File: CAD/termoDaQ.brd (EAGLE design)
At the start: 99.1 x 72.4 mm, 72 parts, among them J1 TEST SUPPLY, J10 POTENTIOMETER, J11 SUPPLY, J12 SUPPLY, J13 V+, J14 B+, J15 VCC, J16 V-, J17 B-, J18 GND, J19 SUPPLY, J2 ADC, J20 VCC, J21 CONN_26X2, J22 CONN_26X2, J23 CONN_26X2, J24 CONN_20X2, J25 FEMALE 2x3, J3 GPS, J4 SERIAL, J5 GPS ON/OF, J6 INT, J7 MPX, J8 SD, J9 EN, T1 2N2222, U1 328P, U2 DS18B20, U3 TINY85-20-DIP, Y1 16MHz, Y2 16MHz

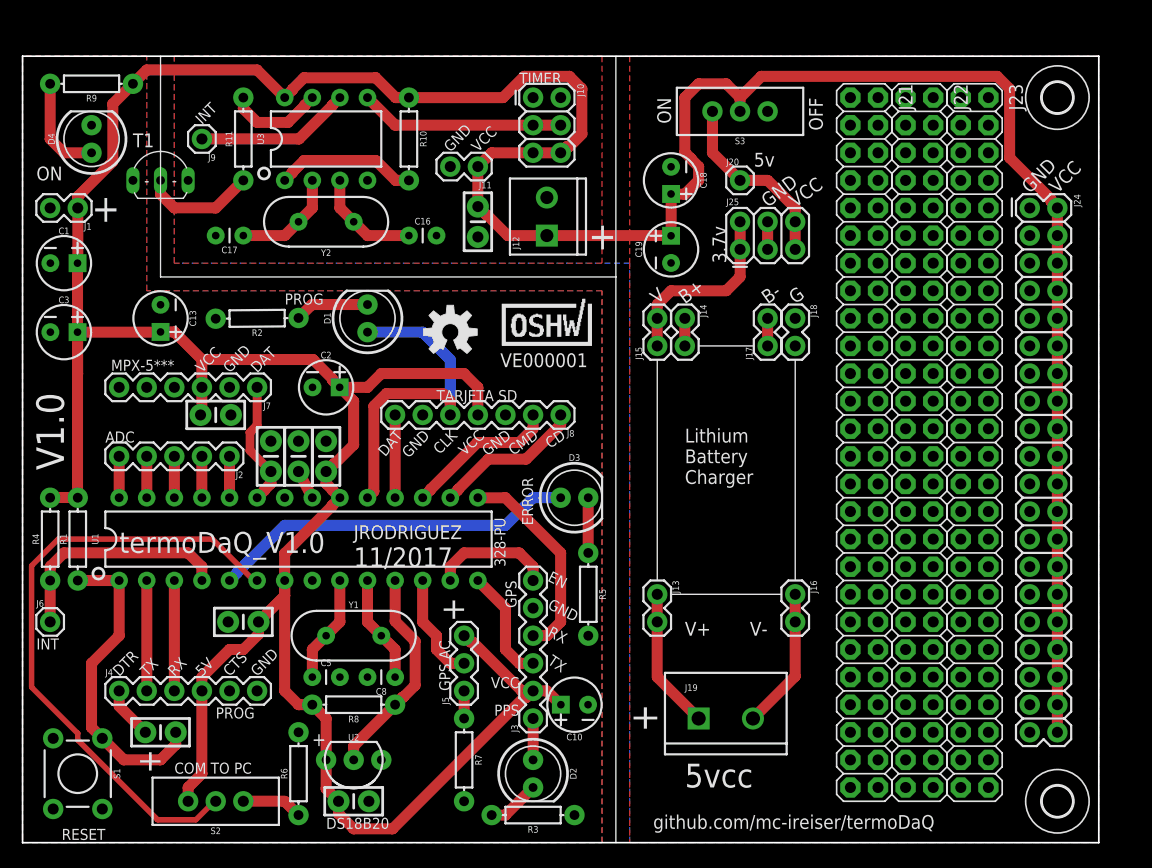
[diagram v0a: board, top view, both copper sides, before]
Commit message: Source files, Update
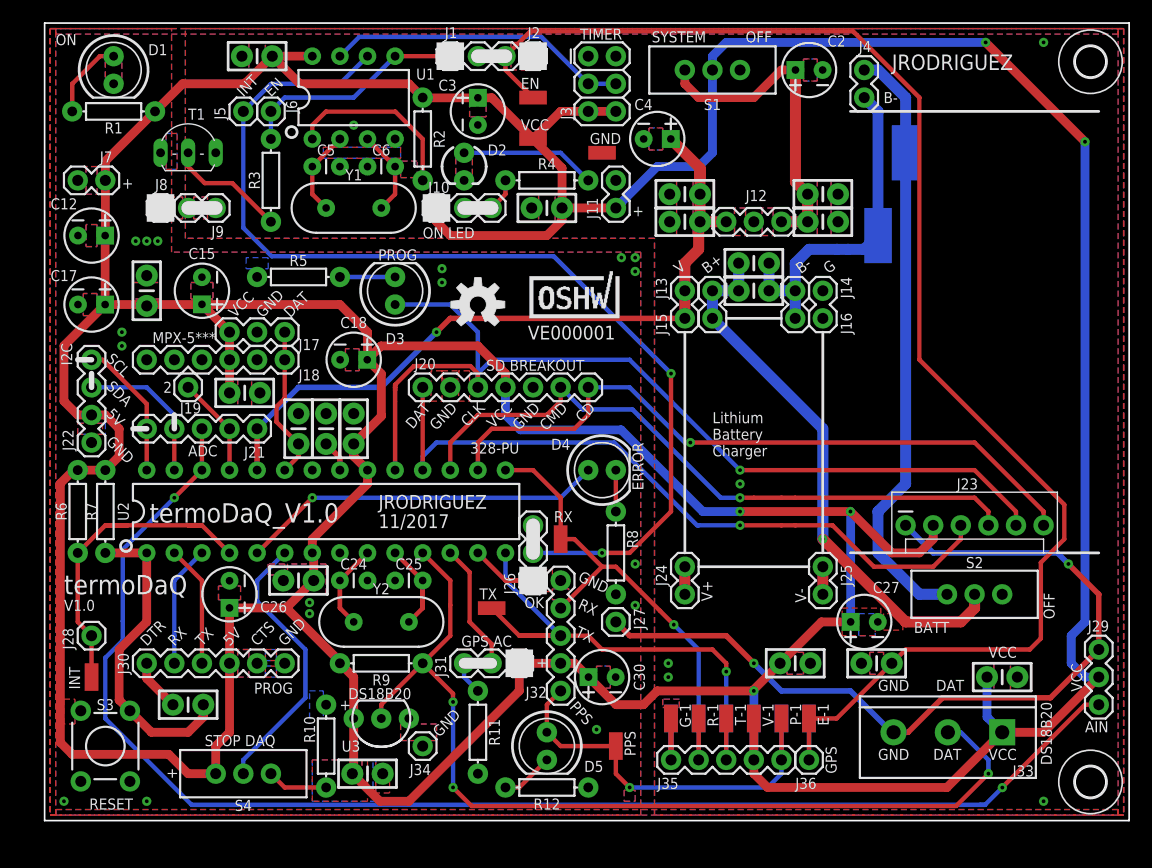
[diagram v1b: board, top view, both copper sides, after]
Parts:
- added B+: B+, wirepad:SMD2,54-5,08
- added B-: B-, wirepad:SMD2,54-5,08
- added C20, C21, C22, C23, C28, C29, C31, C32, C33: 0.1uF, SparkFun-Capacitors:CAP-PTH-SMALL-KIT
- added C24, C25: 22pF, SparkFun-Capacitors:CAP-PTH-2.54
- added C26, C27, C30: 10uF, SparkFun-Capacitors:CPOL-RADIAL-2.5MM-5MM
- added D5: PPS, SparkFun-LED:LED_5MM
- added E-1, E-2, EN: EN GPS, wirepad:SMD1,27-2,54
- added G-1, G-2: G, wirepad:SMD1,27-2,54
- added GND: GND, wirepad:SMD1,27-2,54
- added INT: INT1, wirepad:SMD1,27-2,54
- added J26: OK, SparkFun-Connectors:1X03
- added J27: GND2, SparkFun-Connectors:1X01
- added J28: INT1, SparkFun-Connectors:1X01
- added J29: AIN, SparkFun-Connectors:1X03
- added J30: SERIAL, SparkFun-Connectors:1X06
- added J31: GPS ON/OF, SparkFun-Connectors:1X03
- added J32, J35: GPS, SparkFun-Connectors:1X05
- added J33: TERMINAL SONDA, SparkFun-Connectors:SCREWTERMINAL-5MM-3
- added J34: GND, SparkFun-Connectors:1X01
- added J36: EN, SparkFun-Connectors:1X01
- added P-1, P-2: P, wirepad:SMD1,27-2,54
- added PPS: PPS, wirepad:SMD1,27-2,54
- added R-1, R-2: R, wirepad:SMD1,27-2,54
- added R12: 330, SparkFun-Resistors:AXIAL-0.3
- added RX: RX, wirepad:SMD1,27-2,54
- added S4: STREAM, SparkFun-Switches:SWITCH_SPDT_PTH_11.6X4.0MM
- added T-1, T-2: T, wirepad:SMD1,27-2,54
- added TX: TX, wirepad:SMD1,27-2,54
- added U$100: (no value), SparkFun-Aesthetics:OSHW-LOGO-M
- added U$101: (no value), OSHWA:CERT-SMALL-SILK
- added V-1, V-2: V, wirepad:SMD1,27-2,54
- added VCC: VCC, wirepad:SMD1,27-2,54
- C1, C10, C13, C19: value 22uF -> 0.1uF; device SparkFun-Capacitors:CPOL-RADIAL-2.5MM-5MM -> SparkFun-Capacitors:CAP-PTH-SMALL-KIT
- C12, C15, C4: value 0.1uF -> 10uF; device SparkFun-Capacitors:CAP-PTH-SMALL-KIT -> SparkFun-Capacitors:CPOL-RADIAL-2.5MM-5MM
- C16, C8: value 22pF -> 0.1uF; device SparkFun-Capacitors:CAP-PTH-2.54 -> SparkFun-Capacitors:CAP-PTH-SMALL-KIT
- C17: value 22pF -> 10uF; device SparkFun-Capacitors:CAP-PTH-2.54 -> SparkFun-Capacitors:CPOL-RADIAL-2.5MM-5MM
- C18, C2, C3: value 22uF -> 10uF
- C6: value 0.1uF -> 22pF; device SparkFun-Capacitors:CAP-PTH-SMALL-KIT -> SparkFun-Capacitors:CAP-PTH-2.54
- D1: value PROG -> ON
- D2: value PPS -> POWER; device SparkFun-LED:LED_5MM -> SparkFun-LED:LED_3MM
- D3: value ERROR -> PROG
- D4: value ON -> ERROR
- J1: value TEST SUPPLY -> JUMPER EN; device SparkFun-Connectors:1X02 -> SparkFun-Connectors:1X03
- J10: value POTENTIOMETER -> LED ON/OFF; device SparkFun-Connectors:2X3 -> SparkFun-Connectors:1X03
- J12: value SUPPLY -> STEP UP; device SparkFun-Connectors:SCREWTERMINAL-3.5MM-2 -> SparkFun-Connectors:1X03
- J13: value V+ -> B+
- J14: value B+ -> GND
- J16: value V- -> B-
- J17: value B- -> MPX EXT; device SparkFun-Connectors:1X02 -> SparkFun-Connectors:1X03
- J18: value GND -> MPX; device SparkFun-Connectors:1X02 -> SparkFun-Connectors:1X06
- J19: value SUPPLY -> E_AD2; device SparkFun-Connectors:SCREWTERMINAL-5MM-2 -> SparkFun-Connectors:1X01
- J2: value ADC -> G; device SparkFun-Connectors:1X05 -> SparkFun-Connectors:1X01
- J20: value VCC -> SD; device SparkFun-Connectors:1X01 -> SparkFun-Connectors:1X07
- J21: value CONN_26X2 -> ADC; device SparkFun-Connectors:2X26 -> SparkFun-Connectors:1X05
- J22: value CONN_26X2 -> I2C; device SparkFun-Connectors:2X26 -> SparkFun-Connectors:1X04
- J23: value CONN_26X2 -> MODULO SD; device SparkFun-Connectors:2X26 -> SparkFun-Connectors:MOLEX-1X6
- J24: value CONN_20X2 -> V+; device SparkFun-Connectors:2X20 -> SparkFun-Connectors:1X02
- J25: value FEMALE 2x3 -> V-; device SparkFun-Connectors:2X3 -> SparkFun-Connectors:1X02
- J3: value GPS -> FEMALE 2x3; device SparkFun-Connectors:1X06 -> SparkFun-Connectors:2X3
- J4: value SERIAL -> BETERIA; device SparkFun-Connectors:1X06 -> SparkFun-Connectors:1X02
- J5: value GPS ON/OF -> INT2; device SparkFun-Connectors:1X03 -> SparkFun-Connectors:1X01
- J6: value INT -> EN
- J7: value MPX -> TEST SUPPLY; device SparkFun-Connectors:1X06 -> SparkFun-Connectors:1X02
- J8: value SD -> GND; device SparkFun-Connectors:1X07 -> SparkFun-Connectors:1X01
- J9: value EN -> GND; device SparkFun-Connectors:1X01 -> SparkFun-Connectors:1X02
- R1: value 10k -> 330
- R10: value 4.7k -> 1k
- R2, R3, R9: value 330 -> 1k
- R6: value 1k -> 330
- R7: value 1k -> 10k
- R8: value 4.7k -> 330
- S1: value RESET -> ON/OFF; device SparkFun-Switches:TACTILE_SWITCH_PTH_6.0MM -> SparkFun-Switches:SWITCH_SPDT_PTH_11.6X4.0MM
- S2: value STREAM -> ON/OFF
- S3: value ON/OFF -> RESET; device SparkFun-Switches:SWITCH_SPDT_PTH_11.6X4.0MM -> SparkFun-Switches:TACTILE_SWITCH_PTH_6.0MM
- U$1: device holes:2,8 -> SparkFun-Aesthetics:OSHW-LOGO-M
- U$4: device SparkFun-Aesthetics:OSHW-LOGO-M -> holes:2,8
- U1: value 328P -> TINY85-20-DIP; device SparkFun-IC-Microcontroller:DIP28 -> SparkFun-Retired:DIP08_MCU
- U2: value DS18B20 -> 328P; device SparkFun-Sensors:TO-92-AMMO -> SparkFun-IC-Microcontroller:DIP28
- U3: value TINY85-20-DIP -> DS18B20; device SparkFun-Retired:DIP08_MCU -> SparkFun-Sensors:TO-92-AMMO
- moved J4 89.3 mm to (76.2, 69.8), turned to 270 degrees
- moved S1 87.2 mm to (62.2, 69.8), turned to 90 degrees
- moved S3 82.6 mm to (6.35, 7.62), turned to 270 degrees
- moved J22 78.9 mm to (5.08, 35.6), turned to 90 degrees
- moved S2 72.4 mm to (86.4, 21.6), turned to 270 degrees
- moved U$4 72.0 mm to (97.0, 4.32)
- moved U$1 70.3 mm to (40.6, 48.3)
- moved R3 63.2 mm to (21.6, 59.7), turned to 90 degrees
- moved J3 61.2 mm to (50.8, 71.1), turned to 270 degrees
- moved C8 60.2 mm to (72.4, 58.4), turned to 0 degrees
- moved C9 59.9 mm to (47.0, 57.1), turned to 0 degrees
- moved R9 59.6 mm to (31.8, 15.2)
- moved J21 59.0 mm to (20.3, 36.8), turned to 180 degrees
- moved R11 58.7 mm to (40.6, 8.89), turned to 270 degrees
- moved J5 57.1 mm to (19.1, 66.0), turned to 0 degrees
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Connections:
- removed net AD1: J2.1, U1.24
- removed net N$1: C8.1, U1.10, Y1.2
- removed net N$10: D3.A, U1.5
- removed net N$11: J10.3, J10.4, U3.5
- removed net N$13: J14.1, J14.2
- removed net N$14: C17.1, U3.2, Y2.2
- removed net N$15: R8.P$1, U1.11, U2.2
- removed net N$18: J4.2, U1.2
- removed net N$19: J4.3, U1.3
- removed net N$2: C5.1, U1.9, Y1.1
- removed net N$21: J6.1, R4.P$1, U1.4
- removed net N$22: R11.P$2, U3.7
- removed net N$23: C16.1, U3.3, Y2.1
- removed net N$24: D4.A, R9.P$2
- removed net N$25: J5.2, U1.12
- removed net N$3: C7.2, U1.21
- removed net N$31: J17.1, J17.2
- removed net N$32: J13.1, J13.2, J19.1
- removed net N$33: J16.1, J16.2, J19.2
- removed net N$4: C9.1, R1.P$1, S1.1, U1.1
- removed net N$5 (its old number): D1.K, R2.P$1
- removed net N$6: R10.P$2, U3.1
- removed net N$7: J9.1, U3.6
- removed net N$9: C11.1, J7.1, U1.23
- new net /RESET: C32.1, R7.P$1, S3.1, U2.1
- new net AREF: C21.2, U2.21
- new net B+: C13.1, C16.1, J13.1, J13.2, S2.2
- new net B+IN: B+.1, J4.1, S2.3
- new net B-: B-.1, C13.2, C16.2, J16.1, J16.2, J4.2
- new net DS18B20: J33.2, R9.P$1, U2.11, U3.2
- new net ERROR: D4.A, U2.5
- new net GND2: J23.1, J27.1, J29.1, J33.3
- new net INT1: INT.1, J28.1, R6.P$1, U2.4
- new net INT2: J26.2, J26.3, J5.1, U1.6
- new net JA_LED: J10.2, J10.3, R4.P$1
- new net J_EN: J1.1, J6.1, R3.P$2, U1.5
- new net MPX: C20.1, J17.1, J18.1, U2.23
- new net M_XTAL1: C24.1, U2.9, Y2.1
- new net M_XTAL2: C25.1, U2.10, Y2.2
- new net N$12: D4.K, R8.P$1
- new net NRES: R2.P$2, U1.1
- new net OK: J26.1, U2.13
- new net POT: J3.3, J3.4, U1.7
- new net PWR_LED1: D2.A, R4.P$2
- new net PWR_LED2: D1.A, R1.P$2
- new net R/GPS: J31.2, U2.12
- new net RX: J30.3, U2.2
- new net TX: J30.2, U2.3
- new net V+: J24.1, J24.2
- new net V-: J25.1, J25.2
- new net XTAL1: C6.2, U1.3, Y1.2
- new net XTAL2: C5.1, U1.2, Y1.1
- net 5V: now also C1.2, C12.1, C15.1, C17.1, C19.2, C22.1, C23.2, C26.1, C27.1, C28.1, C30.1, C31.1, C33.1, C9.2, J10.1, J17.3, J18.3, J20.4, J22.2, J23.2, J29.2, J3.5, J3.6, J30.4, J31.3, J32.2, J33.1, J35.2, J7.1, R1.P$1, R2.P$1, R6.P$2, R7.P$2, R9.P$2, S1.2, S4.1, U1.8, U2.20, U2.7, U3.3, V-1.1, V-2.1, VCC.1; no longer C1.1, C10.1, C12.2, C13.1, C15.2, C19.1, C2.1, C4.1, C6.2, J1.1, J10.5, J10.6, J12.1, J24.10, J24.12, J24.14, J24.16, J24.18, J24.2, J24.20, J24.22, J24.24, J24.26, J24.28, J24.30, J24.32, J24.34, J24.36, J24.38, J24.4, J24.40, J24.6, J24.8, J3.2, J4.4, J5.3, J7.3, J8.4, R1.P$2, R10.P$1, R4.P$2, R8.P$2, R9.P$1, S2.1, S3.2, U1.20, U1.7, U2.3, U3.8
- net AD2: now also J19.1, J21.2, U2.25; no longer J2.2, U1.25
- net AD3: now also J21.3, J29.3, U2.26; no longer J2.3, U1.26
- net AD4: now also J21.4, J22.3, U2.27; no longer J2.4, U1.27
- net AD5: now also J21.5, J22.4, U2.28; no longer J2.5, U1.28
- net CD: now also J20.1, J23.6, U2.16; no longer J8.1, U1.16
- net CLK: now also D3.A, J20.5, J23.5, U2.19; no longer D1.A, J8.5, U1.19
- net CMD: now also J20.2, J23.4, U2.17; no longer J8.2, U1.17
- net DAT: now also J20.7, J23.3, U2.18; no longer J8.7, U1.18
- net DTR: now also C32.2, J30.1; no longer C9.2, J4.1
- net EN: now also C29.1, E-1.1, E-2.1, EN.1, J1.2, J1.3, J36.1; no longer J3.6, U1.13
- net GND: now also C1.1, C12.2, C15.2, C19.1, C20.2, C21.1, C22.2, C23.1, C24.2, C25.2, C26.2, C27.2, C28.2, C29.2, C30.2, C31.2, C33.2, C7.2, C9.1, D1.K, D2.K, G-1.1, G-2.1, GND.1, J14.1, J14.2, J17.2, J2.1, J20.3, J20.6, J22.1, J3.1, J3.2, J30.5, J30.6, J32.5, J34.1, J35.5, J8.1, J9.1, J9.2, R10.P$2, R11.P$2, R12.P$1, R8.P$2, S3.3, U1.4, U2.22, U2.8, U3.1; no longer C1.2, C12.1, C13.2, C15.1, C16.2, C19.2, C7.1, D4.K, J1.2, J10.1, J10.2, J18.1, J24.1, J24.11, J24.13, J24.15, J24.17, J24.19, J24.21, J24.23, J24.25, J24.27, J24.29, J24.3, J24.31, J24.33, J24.35, J24.37, J24.39, J24.5, J24.7, J24.9, J25.3, J25.4, J3.5, J4.5, J4.6, J8.3, J8.6, R2.P$2, R3.P$1, R6.P$2, R7.P$2, S1.3, U1.22, U1.8, U2.1, U3.4
- net N$16: now also J31.1, R11.P$1; no longer J5.1, R7.P$1
- net N$17: now also R10.P$1, S4.3; no longer R6.P$1, S2.3
- net N$20: now also R3.P$1; no longer R11.P$1
- net N$8: now also D5.K, R12.P$2; no longer D2.K, R3.P$2
- net PC: now also S4.2, U2.6; no longer S2.2, U1.6
- net PPS: now also D5.A, J32.1, J35.1, P-1.1, P-2.1, PPS.1; no longer D2.A, J3.1
- net R: now also J32.4, J35.4, R-1.1, R-2.1, RX.1, U2.15; no longer J3.4, U1.15
- net T: now also J32.3, J35.3, T-1.1, T-2.1, TX.1, U2.14; no longer J3.3, U1.14
- net VCC: now also C11.1, C2.1, C8.1, J12.3, S1.1; no longer J20.1, J25.5, J25.6, S3.1
- net V_BATT: now also C10.1, C4.1, C7.1, J12.1, J21.1, U2.24; no longer J25.1, J25.2
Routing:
- net 5V: track 393.7 -> 565.4 mm, vias 0 -> 5
- net EN: track 11.2 -> 137.2 mm
- net AD3: track 3.81 -> 129.4 mm, vias 0 -> 2
- net INT2: track 0.00 -> 98.7 mm, vias 0 -> 2
- net DS18B20: track 0.00 -> 88.8 mm, vias 0 -> 3
- net GND2: track 0.00 -> 77.3 mm, vias 0 -> 2
- net CLK: track 31.5 -> 90.4 mm, vias 0 -> 1
- net DAT: track 7.62 -> 66.0 mm, vias 0 -> 1
- net B+IN: track 0.00 -> 55.8 mm
- net V_BATT: track 17.6 -> 68.9 mm, vias 0 -> 1
- net B+: track 0.00 -> 50.9 mm, vias 0 -> 1
- net CD: track 13.9 -> 64.2 mm, vias 0 -> 1
- net CMD: track 14.1 -> 60.9 mm, vias 0 -> 1
- net T: track 10.5 -> 49.9 mm, vias 0 -> 1
- net PPS: track 3.81 -> 38.9 mm, vias 0 -> 1
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- added copper zone on layer 1, net GND-CUT
- added copper zone on layer 16, net GND-CUT
- added copper zone on layer 1, net N$1
- added copper zone on layer 16, net N$10
- added copper zone on layer 16, net N$100
- added copper zone on layer 16, net N$101
- added copper zone on layer 1, net N$102
- added copper zone on layer 1, net N$103
- added copper zone on layer 16, net N$104
- added copper zone on layer 16, net N$105
- added copper zone on layer 1, net N$106
- added copper zone on layer 1, net N$107
- added copper zone on layer 16, net N$108
- added copper zone on layer 1, net N$11
- added copper zone on layer 1, net N$13
- added copper zone on layer 16, net N$14
- added copper zone on layer 1, net N$15
- added copper zone on layer 16, net N$18
- added copper zone on layer 16, net N$19
- added copper zone on layer 1, net N$2
- added copper zone on layer 1, net N$21
- added copper zone on layer 1, net N$22
- added copper zone on layer 16, net N$23
- added copper zone on layer 16, net N$24
- added copper zone on layer 16, net N$25
- added copper zone on layer 1, net N$26
- added copper zone on layer 1, net N$27
- added copper zone on layer 16, net N$28
- added copper zone on layer 1, net N$29
- added copper zone on layer 16, net N$3
- added copper zone on layer 1, net N$30
- added copper zone on layer 16, net N$31
- added copper zone on layer 1, net N$32
- added copper zone on layer 1, net N$33
- added copper zone on layer 16, net N$34
- added copper zone on layer 16, net N$35
- added copper zone on layer 1, net N$36
- added copper zone on layer 1, net N$37
- added copper zone on layer 16, net N$38
- added copper zone on layer 16, net N$39
- added copper zone on layer 16, net N$4
- added copper zone on layer 1, net N$40
- added copper zone on layer 1, net N$41
- added copper zone on layer 16, net N$42
- added copper zone on layer 16, net N$43
- added copper zone on layer 1, net N$44
- added copper zone on layer 1, net N$45
- added copper zone on layer 16, net N$46
- added copper zone on layer 16, net N$47
- added copper zone on layer 1, net N$48
- added copper zone on layer 1, net N$49
- added copper zone on layer 16, net N$50
- added copper zone on layer 16, net N$51
- added copper zone on layer 1, net N$52
- added copper zone on layer 1, net N$53
- added copper zone on layer 16, net N$54
- added copper zone on layer 16, net N$55
- added copper zone on layer 1, net N$56
- added copper zone on layer 1, net N$57
- added copper zone on layer 1, net N$58
- added copper zone on layer 1, net N$59
- added copper zone on layer 1, net N$6
- added copper zone on layer 1, net N$60
- added copper zone on layer 1, net N$61
- added copper zone on layer 16, net N$62
- added copper zone on layer 16, net N$63
- added copper zone on layer 1, net N$64
- added copper zone on layer 1, net N$65
- added copper zone on layer 16, net N$66
- added copper zone on layer 16, net N$67
- added copper zone on layer 16, net N$68
- added copper zone on layer 1, net N$69
- added copper zone on layer 1, net N$7
- added copper zone on layer 1, net N$70
- added copper zone on layer 16, net N$71
- added copper zone on layer 16, net N$72
- added copper zone on layer 1, net N$73
- added copper zone on layer 1, net N$74
- added copper zone on layer 16, net N$79
- added copper zone on layer 16, net N$80
- added copper zone on layer 1, net N$81
- added copper zone on layer 1, net N$82
- added copper zone on layer 1, net N$83
- added copper zone on layer 16, net N$84
- added copper zone on layer 16, net N$85
- added copper zone on layer 1, net N$86
- added copper zone on layer 1, net N$87
- added copper zone on layer 16, net N$88
- added copper zone on layer 16, net N$9
- added copper zone on layer 16, net N$91
- added copper zone on layer 1, net N$93
- added copper zone on layer 1, net N$95
- added copper zone on layer 16, net N$96
- added copper zone on layer 16, net N$97
- added copper zone on layer 1, net N$98
- added copper zone on layer 1, net N$99
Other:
- board size 99.1 x 72.4 mm -> 99.8 x 73.4 mm
- board text added: "2"
- board text added: "AIN"
- board text added: "BATT"
- board text added: "I2C"
- board text added: "Jesus Alfonso Rodriguez Lista"
- board text added: "OK"
- board text added: "ON LED"
- board text added: "SCL"
- board text added: "SD BREAKOUT"
- board text added: "SDA"
- board text added: "STOP DAQ"
- board text added: "SYSTEM"
- board text added: "termoDaQ"
- board text added: "termoDaQ [OSHW] VE000001 By Jesus Alfonso Rodriguez Lista Is licensed under: Creative Commons Attribution-ShareAlike 4.0 International Public License"
- board text removed: "3.7v"
- board text removed: "5v"
- board text removed: "5vcc"
- board text removed: "COM TO PC"
- board text removed: "TARJETA SD"
